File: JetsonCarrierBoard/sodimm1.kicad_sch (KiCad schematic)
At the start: 1 part

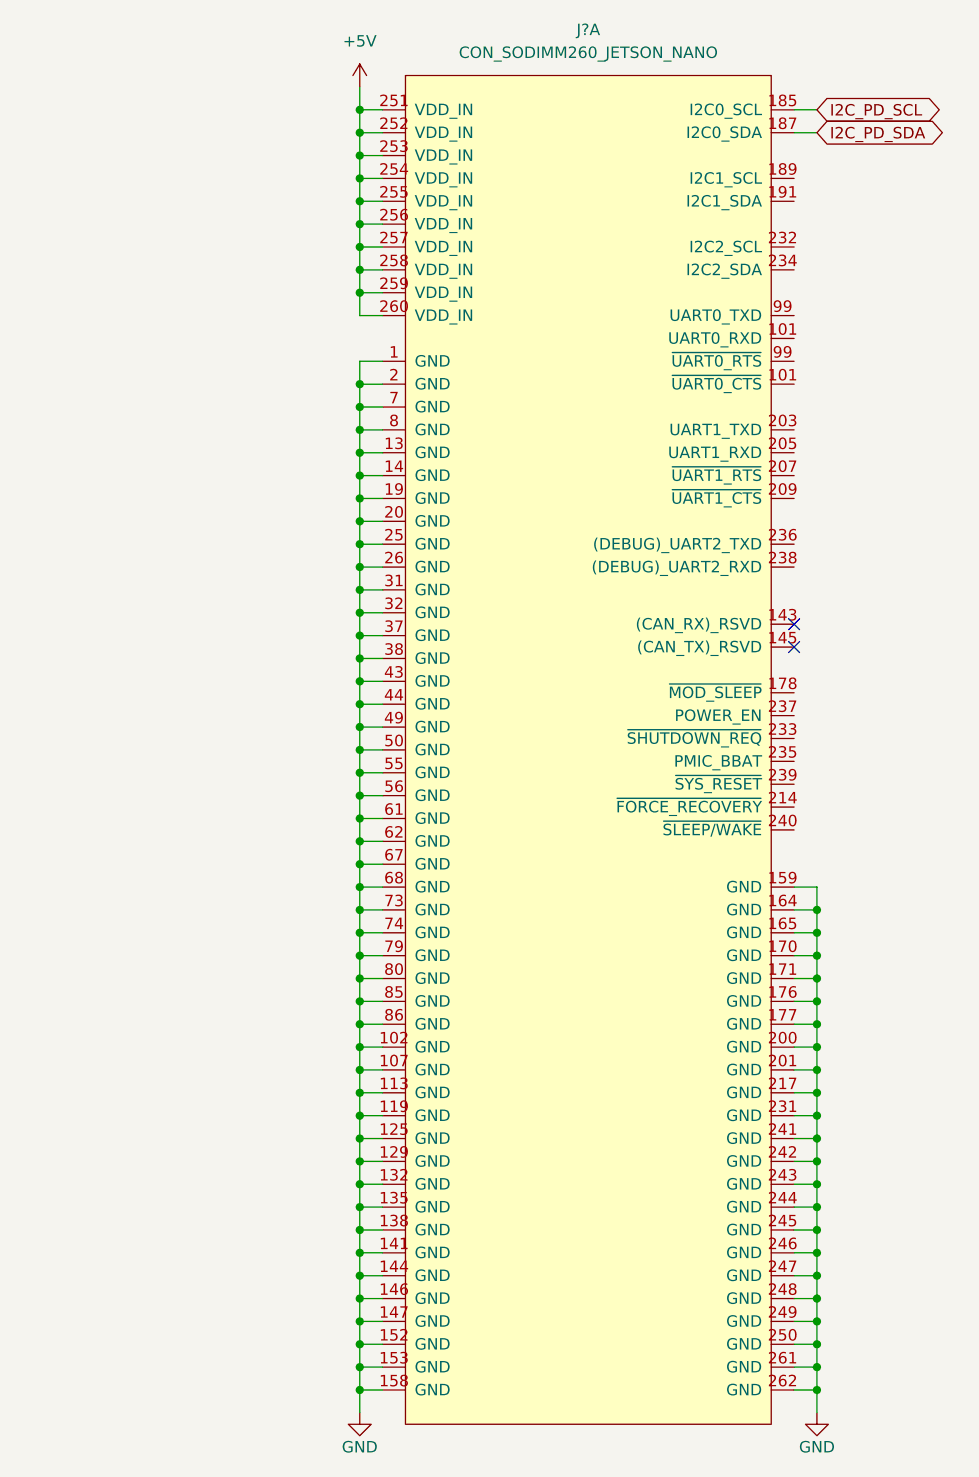
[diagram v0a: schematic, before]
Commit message: Small changes
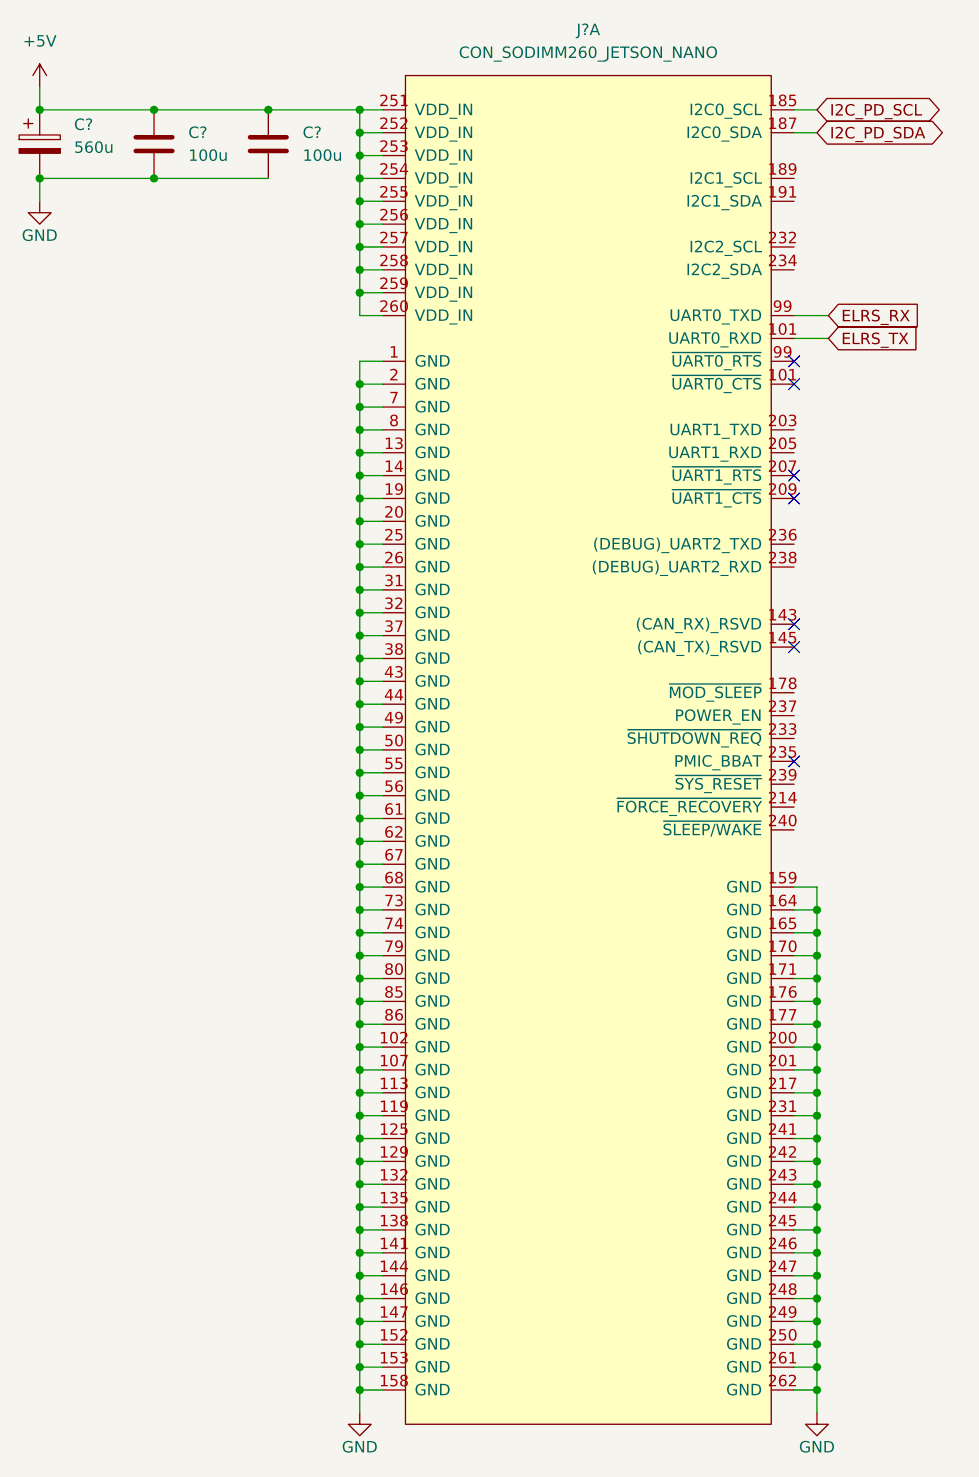
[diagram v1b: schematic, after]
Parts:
- added C?: 560u, symbol Device:C_Polarized
- added C? (x2): 100u, symbol Device:C
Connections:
- net +5V: now also C?.1, C?.1, C?.1
- net GND: now also C?.2, C?.2, C?.2
- net ELRS_TX: now reaches J?.101 (~{UART0_CTS})
- net ELRS_RX: now reaches J?.99 (~{UART0_RTS})
- no-connect marks 2 -> 7
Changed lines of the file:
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@@
   (junction (at 82.55 135.89) (diameter 0) (color 0 0 0 0)
   )
+  (junction (at 59.69 36.83) (diameter 0) (color 0 0 0 0)
+  )
   (junction (at 82.55 29.21) (diameter 0) (color 0 0 0 0)
   )
+  (junction (at 46.99 36.83) (diameter 0) (color 0 0 0 0)
+  )
   (junction (at 82.55 92.71) (diameter 0) (color 0 0 0 0)
   )
   (junction (at 82.55 90.17) (diameter 0) (color 0 0 0 0)
   )
+  (junction (at 72.39 29.21) (diameter 0) (color 0 0 0 0)
+  )
+  (junction (at 59.69 29.21) (diameter 0) (color 0 0 0 0)
+  )
   (junction (at 82.55 87.63) (diameter 0) (color 0 0 0 0)
   )
@@
   (junction (at 82.55 46.99) (diameter 0) (color 0 0 0 0)
   )
+  (junction (at 46.99 29.21) (diameter 0) (color 0 0 0 0)
+  )
   (junction (at 133.35 166.37) (diameter 0) (color 0 0 0 0)
   )
@@
   (junction (at 133.35 125.73) (diameter 0) (color 0 0 0 0)
   )
+  (no_connect (at 130.81 101.6))
+  (no_connect (at 130.81 72.39))
+  (no_connect (at 130.81 69.85))
+  (no_connect (at 130.81 59.69))
+  (no_connect (at 130.81 57.15))
   (no_connect (at 130.81 88.9))
   (no_connect (at 130.81 86.36))
@@
     (stroke (width 0) (type default) (color 0 0 0 0))
   )
+  (wire (pts (xy 59.69 36.83) (xy 72.39 36.83))
+    (stroke (width 0) (type default) (color 0 0 0 0))
+  )
   (wire (pts (xy 85.09 57.15) (xy 82.55 57.15))
     (stroke (width 0) (type default) (color 0 0 0 0))
@@
     (stroke (width 0) (type default) (color 0 0 0 0))
   )
+  (wire (pts (xy 46.99 29.21) (xy 59.69 29.21))
+    (stroke (width 0) (type default) (color 0 0 0 0))
+  )
   (wire (pts (xy 82.55 97.79) (xy 82.55 100.33))
     (stroke (width 0) (type default) (color 0 0 0 0))
@@
     (stroke (width 0) (type default) (color 0 0 0 0))
   )
+  (wire (pts (xy 46.99 36.83) (xy 46.99 39.37))
+    (stroke (width 0) (type default) (color 0 0 0 0))
+  )
+  (wire (pts (xy 130.81 52.07) (xy 134.62 52.07))
+    (stroke (width 0) (type default) (color 0 0 0 0))
+  )
   (wire (pts (xy 82.55 41.91) (xy 85.09 41.91))
     (stroke (width 0) (type default) (color 0 0 0 0))
@@
     (stroke (width 0) (type default) (color 0 0 0 0))
   )
-  (wire (pts (xy 82.55 26.67) (xy 82.55 29.21))
-    (stroke (width 0) (type default) (color 0 0 0 0))
-  )
   (wire (pts (xy 82.55 64.77) (xy 85.09 64.77))
     (stroke (width 0) (type default) (color 0 0 0 0))
@@
     (stroke (width 0) (type default) (color 0 0 0 0))
   )
+  (wire (pts (xy 130.81 54.61) (xy 134.62 54.61))
+    (stroke (width 0) (type default) (color 0 0 0 0))
+  )
   (wire (pts (xy 82.55 166.37) (xy 85.09 166.37))
     (stroke (width 0) (type default) (color 0 0 0 0))
   )
+  (wire (pts (xy 46.99 26.67) (xy 46.99 29.21))
+    (stroke (width 0) (type default) (color 0 0 0 0))
+  )
   (wire (pts (xy 82.55 57.15) (xy 82.55 59.69))
     (stroke (width 0) (type default) (color 0 0 0 0))
@@
     (stroke (width 0) (type default) (color 0 0 0 0))
   )
+  (wire (pts (xy 72.39 29.21) (xy 82.55 29.21))
+    (stroke (width 0) (type default) (color 0 0 0 0))
+  )
   (wire (pts (xy 82.55 135.89) (xy 85.09 135.89))
     (stroke (width 0) (type default) (color 0 0 0 0))
   )
+  (wire (pts (xy 59.69 29.21) (xy 72.39 29.21))
+    (stroke (width 0) (type default) (color 0 0 0 0))
+  )
   (wire (pts (xy 133.35 120.65) (xy 133.35 123.19))
     (stroke (width 0) (type default) (color 0 0 0 0))
@@
   )
   (wire (pts (xy 82.55 163.83) (xy 85.09 163.83))
+    (stroke (width 0) (type default) (color 0 0 0 0))
+  )
+  (wire (pts (xy 46.99 36.83) (xy 59.69 36.83))
     (stroke (width 0) (type default) (color 0 0 0 0))
   )
@@
     (effects (font (size 1.27 1.27)) (justify left))
     (property "Intersheet References" "${INTERSHEET_REFS}" (id 0) (at 146.8302 29.1306 0)
+      (effects (font (size 1.27 1.27)) (justify left) hide)
+    )
+  )
+  (global_label "ELRS_RX" (shape input) (at 134.62 52.07 0) (fields_autoplaced)
+    (effects (font (size 1.27 1.27)) (justify left))
+    (property "Intersheet References" "${INTERSHEET_REFS}" (id 0) (at 145.1369 51.9906 0)
+      (effects (font (size 1.27 1.27)) (justify left) hide)
+    )
+  )
+  (global_label "ELRS_TX" (shape input) (at 134.62 54.61 0) (fields_autoplaced)
+    (effects (font (size 1.27 1.27)) (justify left))
+    (property "Intersheet References" "${INTERSHEET_REFS}" (id 0) (at 144.8345 54.5306 0)
       (effects (font (size 1.27 1.27)) (justify left) hide)
     )
@@
     (pin "98")
   )
+  (symbol (lib_id "power:GND") (at 46.99 39.37 0) (unit 1)
+    (in_bom yes) (on_board yes)
+    (property "Reference" "#PWR?" (id 0) (at 46.99 45.72 0)
+      (effects (font (size 1.27 1.27)) hide)
+    )
+    (property "Value" "GND" (id 1) (at 46.99 43.18 0))
+    (property "Footprint" "" (id 2) (at 46.99 39.37 0)
+      (effects (font (size 1.27 1.27)) hide)
+    )
+    (property "Datasheet" "" (id 3) (at 46.99 39.37 0)
+      (effects (font (size 1.27 1.27)) hide)
+    )
+    (pin "1")
+  )
+  (symbol (lib_id "Device:C_Polarized") (at 46.99 33.02 0) (unit 1)
+    (in_bom yes) (on_board yes) (fields_autoplaced)
+    (property "Reference" "C?" (id 0) (at 50.8 30.8609 0)
+      (effects (font (size 1.27 1.27)) (justify left))
+    )
+    (property "Value" "560u" (id 1) (at 50.8 33.4009 0)
+      (effects (font (size 1.27 1.27)) (justify left))
+    )
+    (property "Footprint" "" (id 2) (at 47.9552 36.83 0)
+      (effects (font (size 1.27 1.27)) hide)
+    )
+    (property "Datasheet" "~" (id 3) (at 46.99 33.02 0)
+      (effects (font (size 1.27 1.27)) hide)
+    )
+    (pin "1")
+    (pin "2")
+  )
+  (symbol (lib_id "Device:C") (at 59.69 33.02 0) (unit 1)
+    (in_bom yes) (on_board yes) (fields_autoplaced)
+    (property "Reference" "C?" (id 0) (at 63.5 31.7499 0)
+      (effects (font (size 1.27 1.27)) (justify left))
+    )
+    (property "Value" "100u" (id 1) (at 63.5 34.2899 0)
+      (effects (font (size 1.27 1.27)) (justify left))
+    )
+    (property "Footprint" "" (id 2) (at 60.6552 36.83 0)
+      (effects (font (size 1.27 1.27)) hide)
+    )
+    (property "Datasheet" "~" (id 3) (at 59.69 33.02 0)
+      (effects (font (size 1.27 1.27)) hide)
+    )
+    (pin "1")
+    (pin "2")
+  )
   (symbol (lib_id "power:GND") (at 133.35 173.99 0) (unit 1)
     (in_bom yes) (on_board yes)
@@
     (pin "1")
   )
-  (symbol (lib_id "power:+5V") (at 82.55 26.67 0) (unit 1)
+  (symbol (lib_id "Device:C") (at 72.39 33.02 0) (unit 1)
     (in_bom yes) (on_board yes) (fields_autoplaced)
-    (property "Reference" "#PWR?" (id 0) (at 82.55 30.48 0)
-      (effects (font (size 1.27 1.27)) hide)
-    )
-    (property "Value" "+5V" (id 1) (at 82.55 21.59 0))
-    (property "Footprint" "" (id 2) (at 82.55 26.67 0)
-      (effects (font (size 1.27 1.27)) hide)
-    )
-    (property "Datasheet" "" (id 3) (at 82.55 26.67 0)
-      (effects (font (size 1.27 1.27)) hide)
-    )
+    (property "Reference" "C?" (id 0) (at 76.2 31.7499 0)
+      (effects (font (size 1.27 1.27)) (justify left))
+    )
+    (property "Value" "100u" (id 1) (at 76.2 34.2899 0)
+      (effects (font (size 1.27 1.27)) (justify left))
+    )
+    (property "Footprint" "" (id 2) (at 73.3552 36.83 0)
+      (effects (font (size 1.27 1.27)) hide)
+    )
+    (property "Datasheet" "~" (id 3) (at 72.39 33.02 0)
+      (effects (font (size 1.27 1.27)) hide)
+    )
+    (pin "1")
+    (pin "2")
+  )
+  (symbol (lib_id "power:+5V") (at 46.99 26.67 0) (unit 1)
+    (in_bom yes) (on_board yes) (fields_autoplaced)
+    (property "Reference" "#PWR?" (id 0) (at 46.99 30.48 0)
+      (effects (font (size 1.27 1.27)) hide)
+    )
+    (property "Value" "+5V" (id 1) (at 46.99 21.59 0))
+    (property "Footprint" "" (id 2) (at 46.99 26.67 0)
+      (effects (font (size 1.27 1.27)) hide)
+    )
+    (property "Datasheet" "" (id 3) (at 46.99 26.67 0)
+      (effects (font (size 1.27 1.27)) hide)
+    )
